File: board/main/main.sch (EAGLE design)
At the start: 30 parts, among them IC1 78m05, U1 24LC256, U2 6N138M

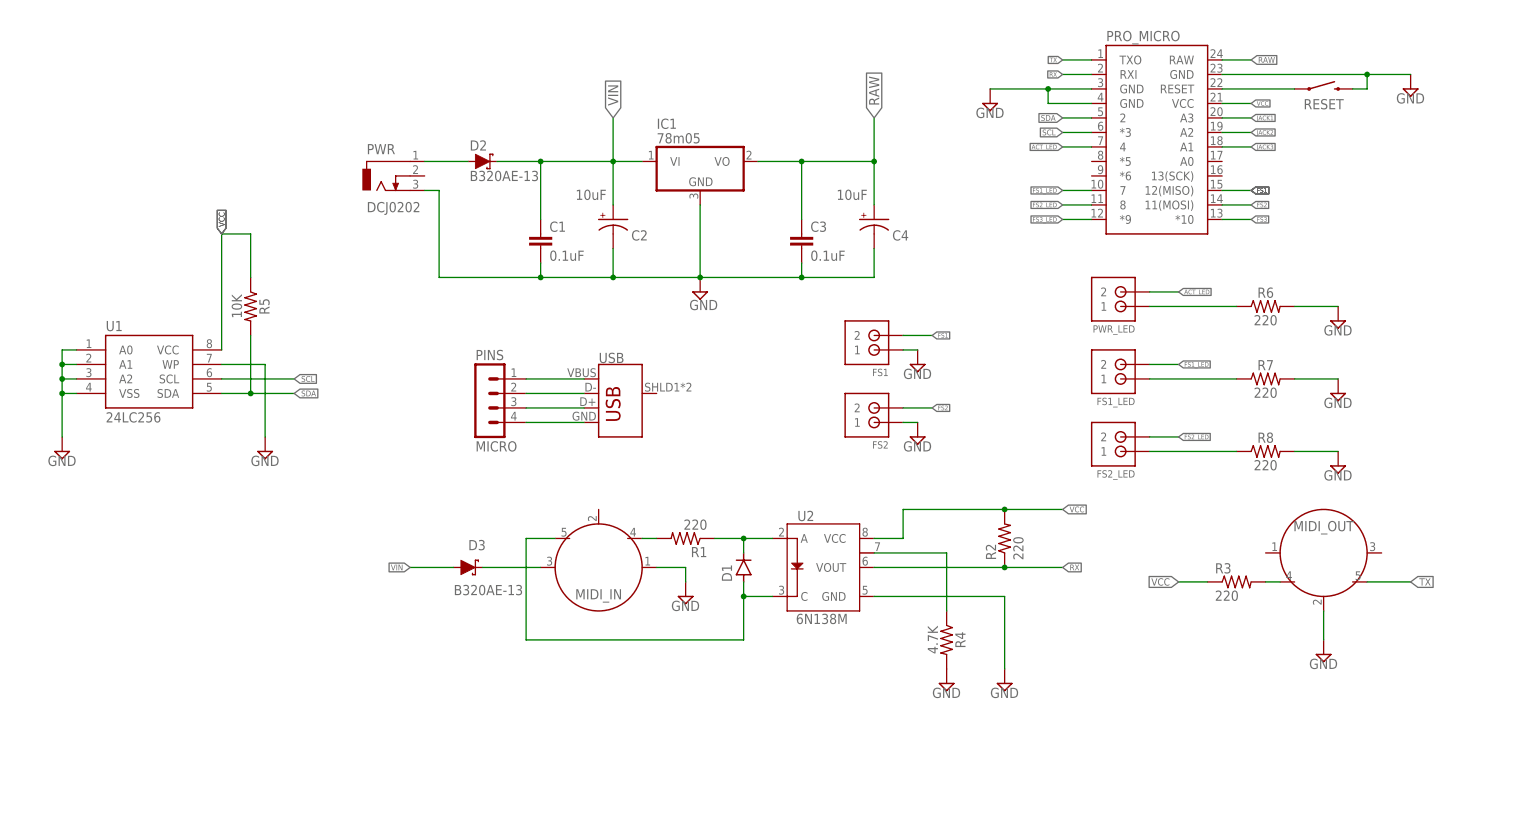
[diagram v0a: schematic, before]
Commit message: latest board changes
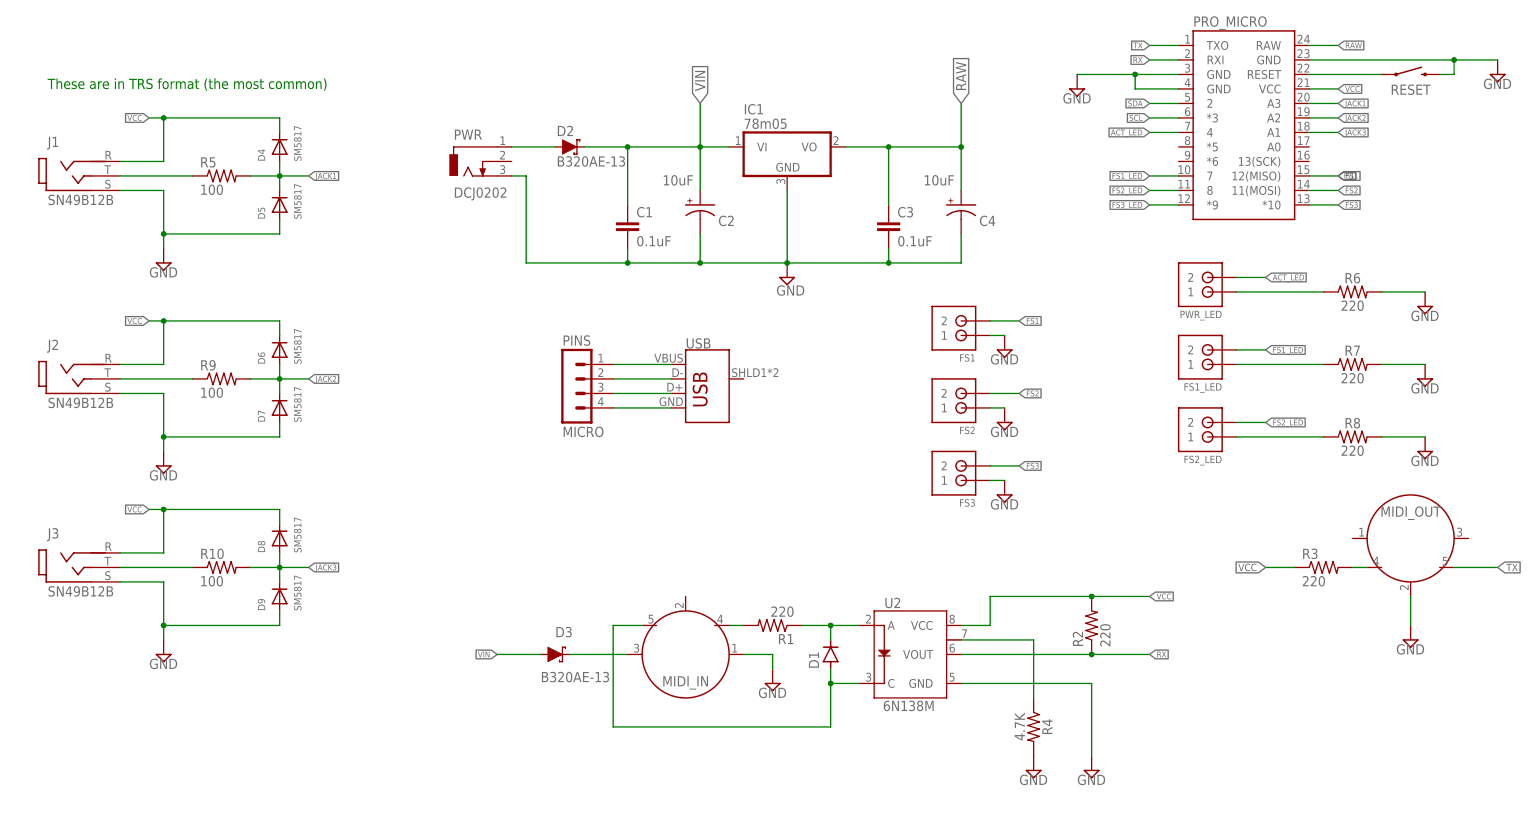
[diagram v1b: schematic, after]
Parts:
- removed U1: 24LC256, SparkFun-IC-Memory:EEPROM-I2CSMD
- added D4, D5, D6, D7, D8, D9: SM5817, adafruit:DIODE_SOD-123FL
- added FS3: JST-PH_2-PIN_HEADER, SRG:JST-PH_2-PIN_HEADER
- added J1, J2, J3: SN49B12B, SN49B12B:SN49B12B
- added R10, R9: 100, SparkFun-Resistors:RESISTOR1206
- R5: value 10K -> 100
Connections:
- new net N$14: J1.T, R5.1
- new net N$9: J2.T, R9.1
- net FS3: now also FS3.2
- net GND: now also D5.A, D7.A, D9.A, FS3.1, J1.S, J2.S, J3.S; no longer U1.A0, U1.A1, U1.A2, U1.VSS, U1.WP
- net JACK1: now also D4.A, D5.C, R5.2
- net JACK2: now also D6.A, D7.C, R9.2
- net JACK3: now also D8.A, D9.C, R10.2
- net N$12: now also J3.T, R10.1; no longer R5.1, U1.VCC
- net SCL: no longer U1.SCL
- net SDA: no longer R5.2, U1.SDA
- net VCC: now also D4.C, D6.C, D8.C, J1.R, J2.R, J3.R
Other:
- note added: "These are in TRS format (the most common)"
- moved on the sheet: C1, C2, C3, C4, D1, D2, D3, FS1, FS1_LED, FS2, FS2_LED, IC1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

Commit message: schematic updates
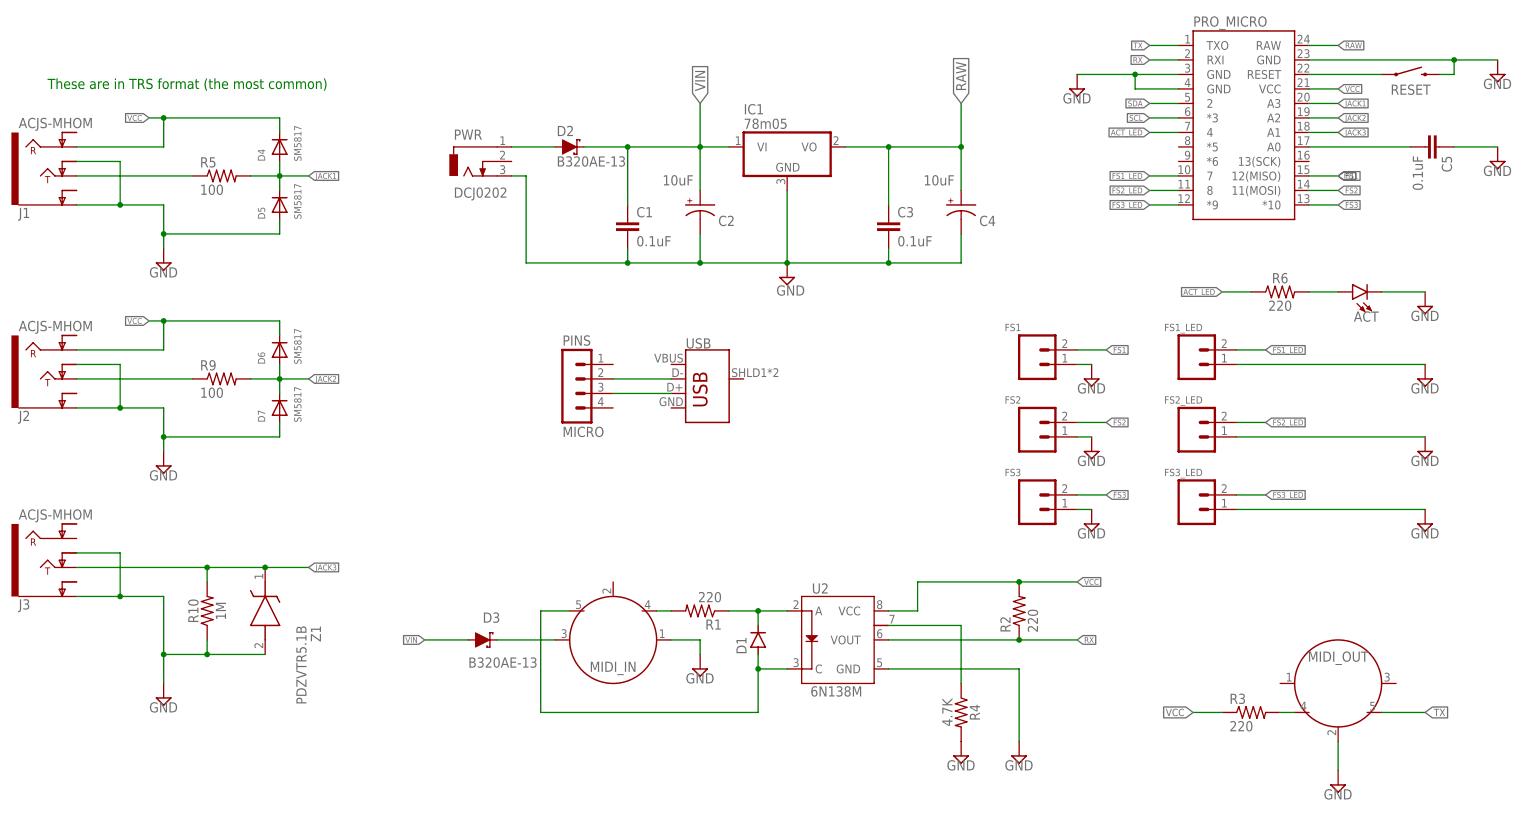
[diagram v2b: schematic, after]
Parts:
- removed D8, D9: SM5817, adafruit:DIODE_SOD-123FL
- removed PWR_LED: JST-PH_2-PIN_HEADER, SRG:JST-PH_2-PIN_HEADER
- removed R7, R8: 220, SparkFun-Resistors:RESISTOR1206
- added ACT: (no value), SparkFun-LED:LED3MM
- added C5: 0.1uF, resistor:C-EUC1206
- added FS3_LED: (no value), SparkFun-Connectors:CONN_02
- added Z1: PDZVTR5.1B, zener:PDZVTR3.0B
- FS1, FS1_LED, FS2, FS2_LED, FS3: value JST-PH_2-PIN_HEADER -> (none); device SRG:JST-PH_2-PIN_HEADER -> SparkFun-Connectors:CONN_02
- J1, J2, J3: value SN49B12B -> ACJS-MHOM; device SN49B12B:SN49B12B -> ACJS-MHOM:ACJS-MHOM
- R10: value 100 -> 1M
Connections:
- removed net N$12: J3.T, R10.1
- removed net N$4: FS1_LED.1, R7.1
- removed net N$6: FS2_LED.1, R8.1
- removed net USB_GND: MICRO.4, USB.GND
- removed net VBUS: MICRO.1, USB.VBUS
- new net N$15: C5.2, PRO_MICRO.A0
- net ACT_LED: now also R6.1; no longer PWR_LED.2
- net FS3_LED: now also FS3_LED.2
- net GND: now also ACT.C, C5.1, FS1_LED.1, FS2_LED.1, FS3_LED.1, J1.EARTH, J1.TIP-NORM, J2.EARTH, J2.TIP-NORM, J3.EARTH, J3.TIP-NORM, R10.1, Z1.A; no longer D9.A, J1.S, J2.S, J3.S, R6.2, R7.2, R8.2
- net JACK3: now also J3.TIP, Z1.K; no longer D8.A, D9.C
- net N$1: now also ACT.A, R6.2; no longer PWR_LED.1, R6.1
- net N$14: now also J1.TIP; no longer J1.T
- net N$9: now also J2.TIP; no longer J2.T
- net VCC: now also J1.RING, J2.RING; no longer D8.C, J1.R, J2.R, J3.R
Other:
- moved on the sheet: D1, D3, FS1, FS1_LED, FS2, FS2_LED, FS3, MIDI_IN, MIDI_OUT, R1, R10, R2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
